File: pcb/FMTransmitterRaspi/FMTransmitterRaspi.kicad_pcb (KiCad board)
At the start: 2 copper layers, 65 x 30 mm, 5 parts, among them J1 GPIO

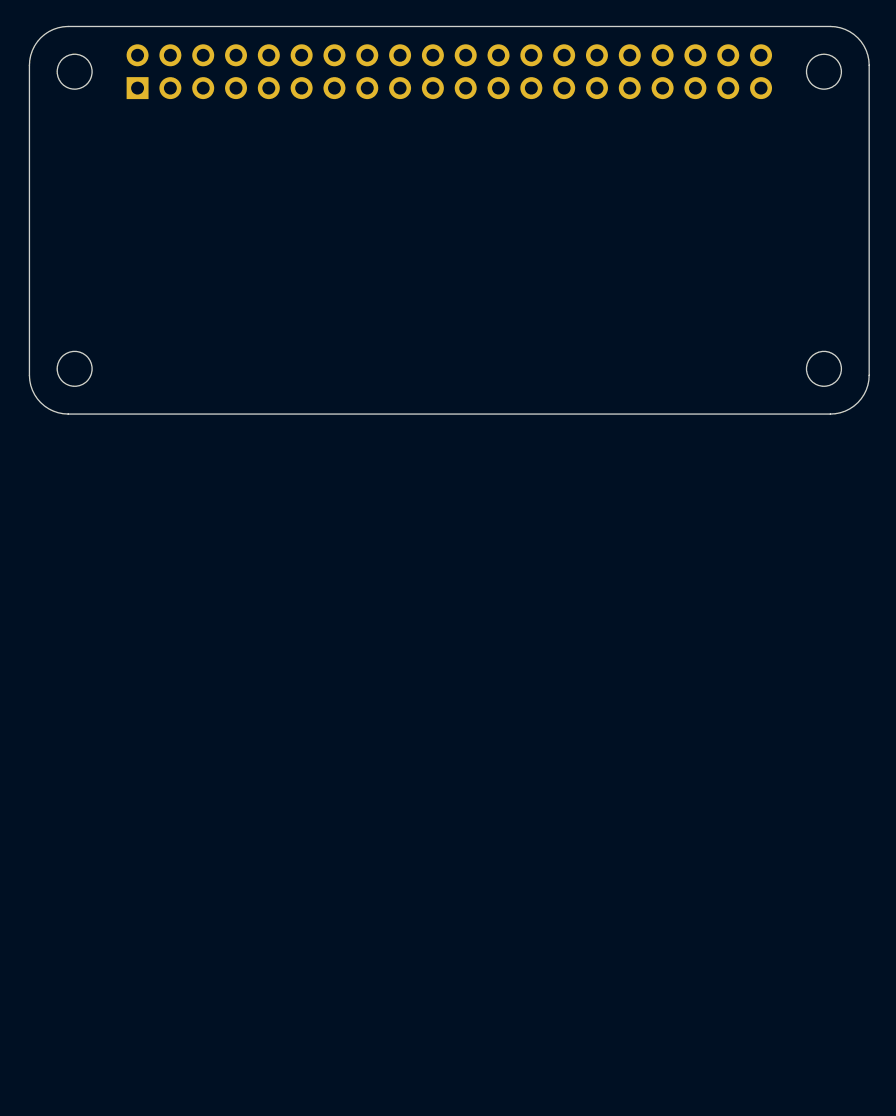
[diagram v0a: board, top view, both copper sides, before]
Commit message: Ready for production
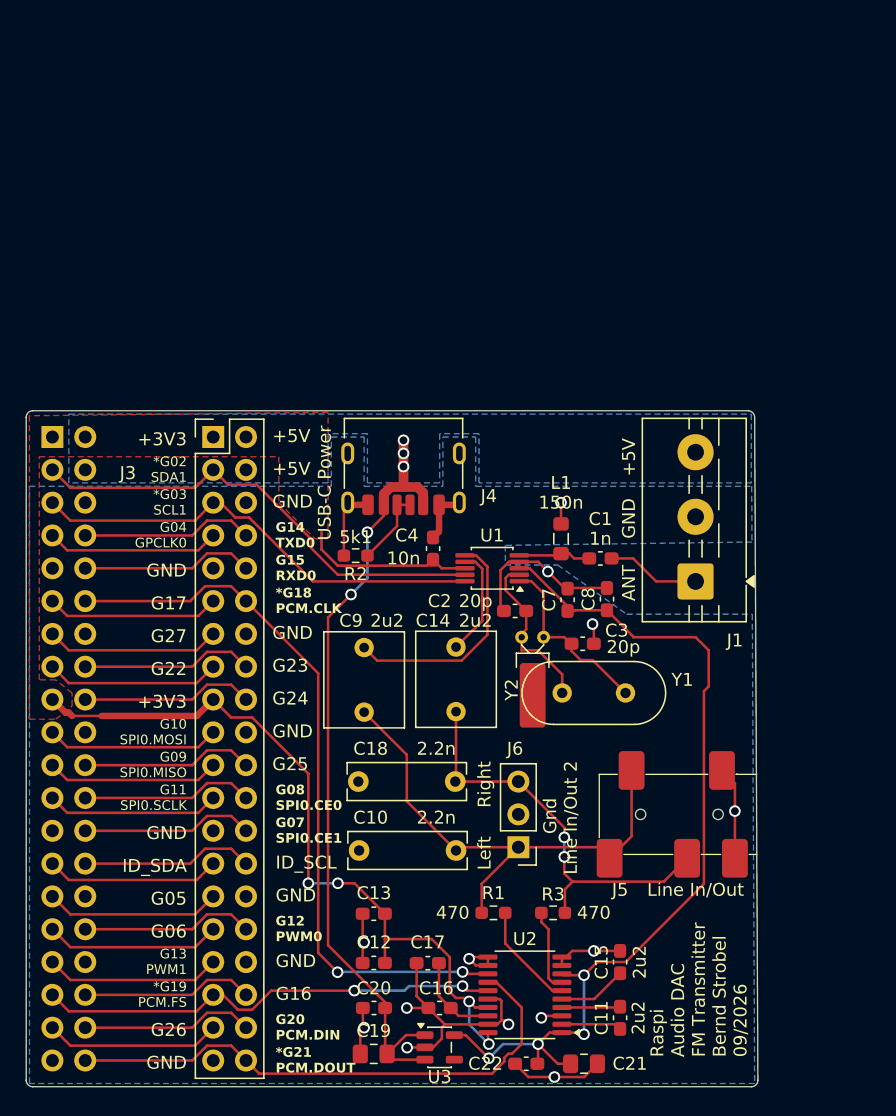
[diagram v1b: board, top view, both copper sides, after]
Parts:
- removed MH1, MH2, MH3, MH4: MountingHole_2.7mm_M2.5, MountingHole:MountingHole_2.7mm_M2.5
- added C1: 1n, Capacitor_SMD:C_0603_1608Metric_Pad1.08x0.95mm_HandSolder, F.Cu at (144.2, 111.2)
- added C10: 2.2n, Capacitor_THT:C_Rect_L9.0mm_W2.7mm_P7.50mm_MKT, F.Cu at (133.0, 133.8)
- added C11: 2u2, Capacitor_SMD:C_0603_1608Metric_Pad1.08x0.95mm_HandSolder, F.Cu at (145.7, 146.7)
- added C12: 10u, Capacitor_SMD:C_0603_1608Metric_Pad1.08x0.95mm_HandSolder, F.Cu at (126.7, 142.5)
- added C13: 100n, Capacitor_SMD:C_0603_1608Metric_Pad1.08x0.95mm_HandSolder, F.Cu at (126.7, 138.7)
- added C14: 2u2, Capacitor_THT:C_Rect_L7.2mm_W6.0mm_P5.00mm, F.Cu at (133.0, 123.0)
- added C15: 2u2, Capacitor_SMD:C_0603_1608Metric_Pad1.08x0.95mm_HandSolder, F.Cu at (145.7, 142.4)
- added C16: 10u, Capacitor_SMD:C_0603_1608Metric_Pad1.08x0.95mm_HandSolder, F.Cu at (131.8, 146.0)
- added C17: 100n, Capacitor_SMD:C_0603_1608Metric_Pad1.08x0.95mm_HandSolder, F.Cu at (130.8, 142.5)
- added C18: 2.2n, Capacitor_THT:C_Rect_L9.0mm_W2.7mm_P7.50mm_MKT, F.Cu at (133.0, 128.4)
- added C19: 10u, Capacitor_SMD:C_0805_2012Metric_Pad1.18x1.45mm_HandSolder, F.Cu at (126.6, 149.5)
- added C2: 20p, Capacitor_SMD:C_0603_1608Metric_Pad1.08x0.95mm_HandSolder, F.Cu at (137.6, 115.2)
- added C20: 100n, Capacitor_SMD:C_0603_1608Metric_Pad1.08x0.95mm_HandSolder, F.Cu at (126.7, 146.0)
- added C21: 10u, Capacitor_SMD:C_0805_2012Metric_Pad1.18x1.45mm_HandSolder, F.Cu at (142.9, 150.3)
- added C22: 100n, Capacitor_SMD:C_0603_1608Metric_Pad1.08x0.95mm_HandSolder, F.Cu at (138.5, 150.3)
- added C3: 20p, Capacitor_SMD:C_0603_1608Metric_Pad1.08x0.95mm_HandSolder, F.Cu at (142.8, 117.8)
- added C4: 10n, Capacitor_SMD:C_0603_1608Metric_Pad1.08x0.95mm_HandSolder, F.Cu at (131.2, 110.4)
- added C7: 10u, Capacitor_SMD:C_0603_1608Metric_Pad1.08x0.95mm_HandSolder, F.Cu at (141.7, 114.4)
- added C8: 100n, Capacitor_SMD:C_0603_1608Metric_Pad1.08x0.95mm_HandSolder, F.Cu at (144.7, 114.3)
- added C9: 2u2, Capacitor_THT:C_Rect_L7.2mm_W6.0mm_P5.00mm, F.Cu at (125.9, 123.1)
- added J1: Antenna/External Power, TerminalBlock:TerminalBlock_MaiXu_MX126-5.0-03P_1x03_P5.00mm, F.Cu at (151.6, 113.0)
- added J3: GPIO, Connector_PinHeader_2.54mm:PinHeader_2x20_P2.54mm_Vertical, F.Cu at (114.2, 101.8)
- added J4: USB-C Power, Connector_USB:USB_C_Receptacle_HRO_TYPE-C-31-M-17, F.Cu at (129.0, 103.8)
- added J5: Line In/Out, Library:Jack_3.5mm_PJ327A_Horizontal, F.Cu at (156.3, 131.0)
- added J6: Line In/Out 2, Connector_PinHeader_2.54mm:PinHeader_1x03_P2.54mm_Vertical, F.Cu at (137.8, 133.5)
- added L1: 150n, Inductor_SMD:L_0805_2012Metric_Pad1.05x1.20mm_HandSolder, F.Cu at (141.1, 109.7)
- added R1: 470, Resistor_SMD:R_0603_1608Metric_Pad0.98x0.95mm_HandSolder, F.Cu at (135.9, 138.6)
- added R2: 5k1, Resistor_SMD:R_0603_1608Metric_Pad0.98x0.95mm_HandSolder, F.Cu at (125.3, 111.0)
- added R3: 470, Resistor_SMD:R_0603_1608Metric_Pad0.98x0.95mm_HandSolder, F.Cu at (140.5, 138.6)
- added U1: QN8072, Package_SO:MSOP-10_3x3mm_P0.5mm, F.Cu at (135.8, 111.9)
- added U2: PCM5102A, Package_SO:TSSOP-20_4.4x6.5mm_P0.65mm, F.Cu at (138.4, 145.0)
- added U3: ME6211C33M5, Package_TO_SOT_SMD:SOT-23-5, F.Cu at (131.8, 149.0)
- added Y1: 24MHz, Crystal:Crystal_HC18-U_Vertical, F.Cu at (146.1, 121.6)
- added Y2: 12MHz, Crystal:Crystal_DS15_D1.5mm_L5.0mm_Horizontal_1EP_style1, F.Cu at (138.1, 117.3)
- J2: renamed from J1; footprint Connector_PinSocket_2.54mm:PinSocket_2x20_P2.54mm_Vertical -> Library:PinSocket_2x20_P2.54mm_Vertical
- moved J2 27.8 mm to (101.8, 101.8), turned to 180 degrees
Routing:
- net GND: track 0.00 -> 78.8 mm, vias 0 -> 13
- net +3V3: track 0.00 -> 72.6 mm, vias 0 -> 4
- net +3.3VA: track 0.00 -> 70.7 mm, vias 0 -> 4
- net +5V: track 0.00 -> 61.7 mm, vias 0 -> 5
- net /GPIO18/PCM.CLK: track 0.00 -> 57.0 mm, vias 0 -> 2
- net /GPIO21/PCM.DOUT: track 0.00 -> 42.5 mm
- net Net-(J6-Pin_1): track 0.00 -> 39.8 mm
- net /GPIO2/SDA1: track 0.00 -> 36.9 mm
- net /GPIO19/PCM.FS: track 0.00 -> 36.1 mm, vias 0 -> 2
- net /GPIO3/SCL1: track 0.00 -> 35.6 mm
- net Net-(J6-Pin_3): track 0.00 -> 32.1 mm, vias 0 -> 2
- net Net-(U1-ALI): track 0.00 -> 18.2 mm
- net Net-(U1-XTAL2): track 0.00 -> 14.1 mm
- net /GPIO6: track 0.00 -> 13.6 mm
- net /GPIO5: track 0.00 -> 13.6 mm
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- added copper zone on F.Cu, net +3V3
- added copper zone on B.Cu, net +5V
- added copper zone on B.Cu, net GND
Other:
- board size 65 x 30 mm -> 56.6 x 52.3 mm
- board text added: "*G02 SDA1"
- board text added: "*G03 SCL1"
- board text added: "*G18 PCM.CLK"
- board text added: "*G19 PCM.FS"
- board text added: "*G21 PCM.DOUT"
- board text added: "+3V3"
- board text added: "+5V"
- board text added: "ANT"
- board text added: "G04 GPCLK0"
- board text added: "G05"
- board text added: "G06"
- board text added: "G07 SPI0.CE1"
- board text added: "G08 SPI0.CE0"
- board text added: "G09 SPI0.MISO"
- board text added: "G10 SPI0.MOSI"
- board text added: "G11 SPI0.SCLK"
- board text added: "G12 PWM0"
- board text added: "G13 PWM1"
- board text added: "G14 TXD0"
- board text added: "G15 RXD0"
- board text added: "G16"
- board text added: "G17"
- board text added: "G20 PCM.DIN"
- board text added: "G22"
- board text added: "G23"
- board text added: "G24"
- board text added: "G25"
- board text added: "G26"
- board text added: "G27"
- board text added: "GND"
- board text added: "Gnd"
- board text added: "ID_SCL"
- board text added: "ID_SDA"
- board text added: "Left"
- board text added: "Raspi Audio DAC FM Transmitter Bernd Strobel 09/2026"
- board text added: "Right"
- board text removed: "Extend PCB edge 0.5mm if using SMT header"
- board text removed: "PoE"
